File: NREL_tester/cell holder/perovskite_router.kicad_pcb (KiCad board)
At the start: 2 copper layers, 38.4 x 45.1 mm, 9 parts, among them J1 Conn_01x10_Male, J2 Conn_01x10_Male, U1 Perovskite_CP_6_Cell, U2 MCP9808_MSOP

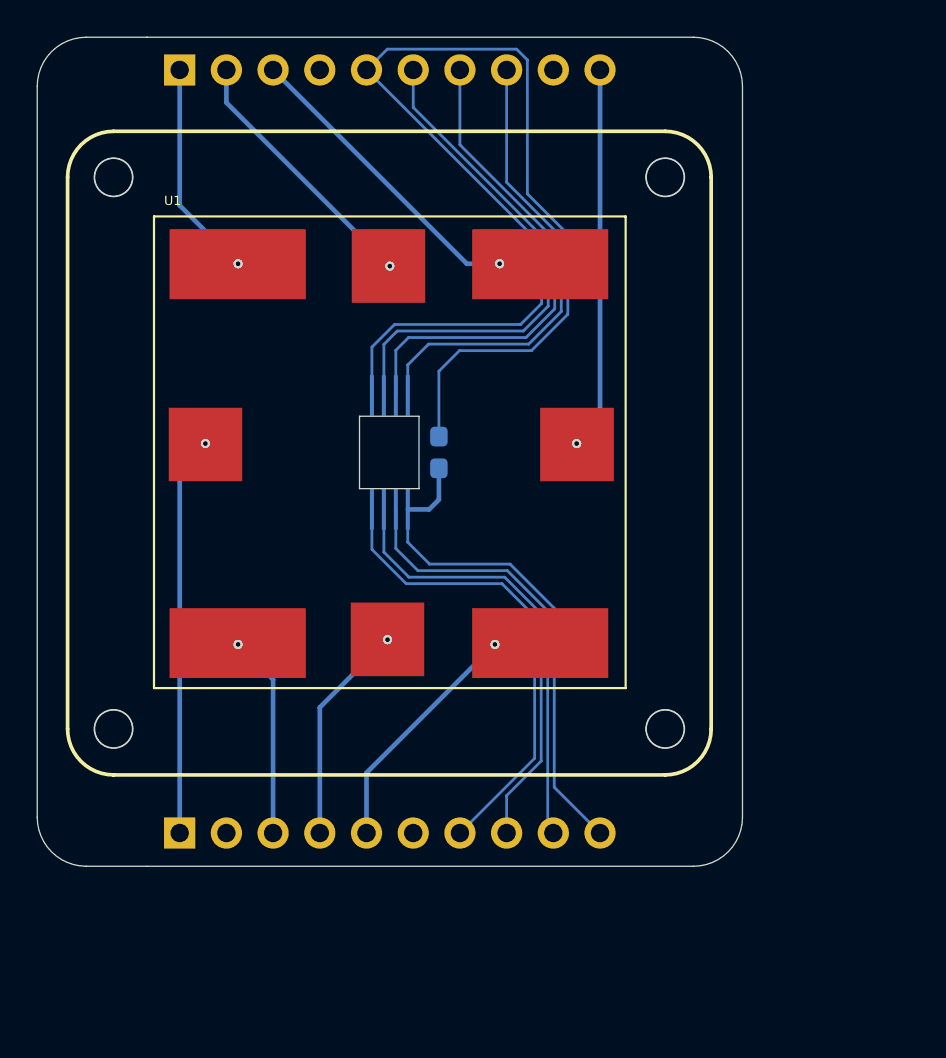
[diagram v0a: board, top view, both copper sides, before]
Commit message: Review contact board
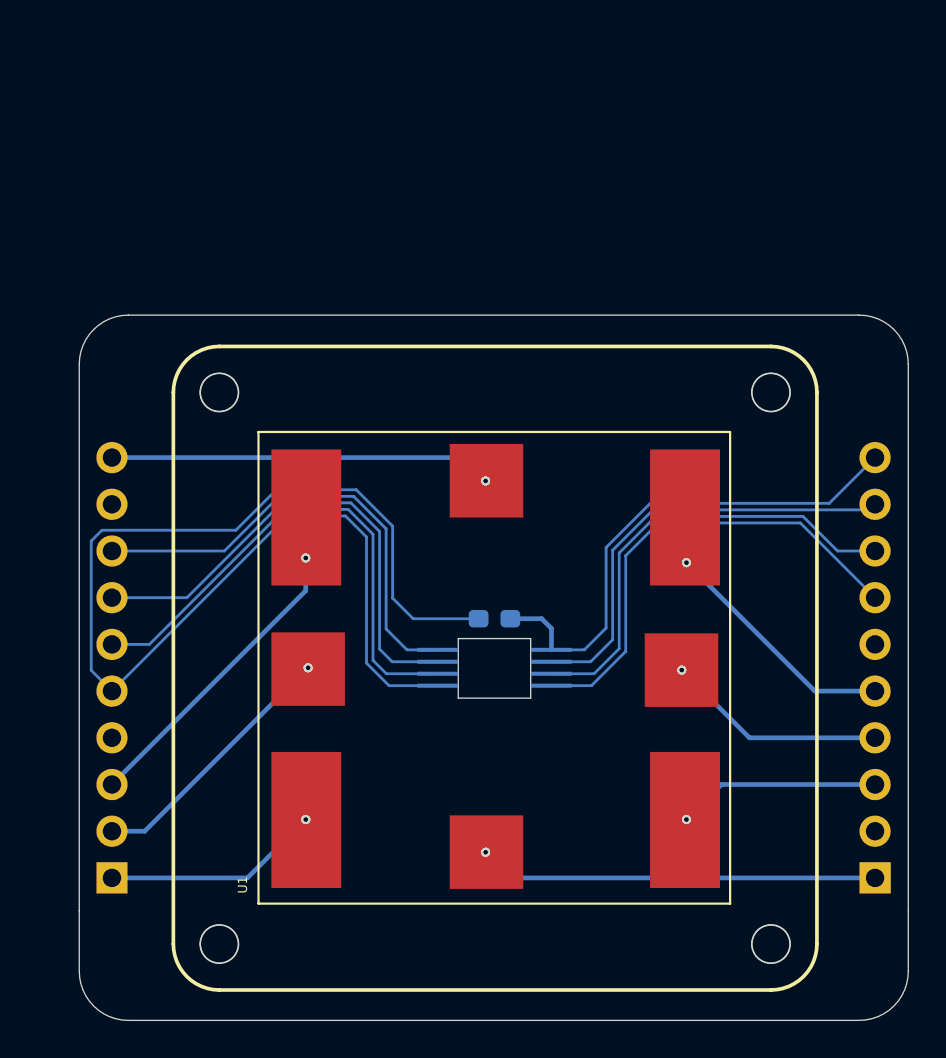
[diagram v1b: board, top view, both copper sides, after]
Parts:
- moved J1 44.1 mm to (134.4, 109.2), turned to 0 degrees
- moved REF** 42.1 mm to (140.2, 112.8), turned to 90 degrees
- moved J2 37.9 mm to (175.9, 109.2), turned to 0 degrees
- moved U1 37.8 mm to (142.3, 110.6), turned to 90 degrees
- moved REF** 37.6 mm to (170.2, 112.8), turned to 90 degrees
- moved REF** 26.9 mm to (140.2, 82.8), turned to 90 degrees
- moved REF** 19.2 mm to (170.2, 82.8), turned to 90 degrees
- moved U2 13.0 mm to (155.2, 97.8), turned to 180 degrees
- moved C1 9.53 mm to (155.2, 95.1), turned to 180 degrees
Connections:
- net Net-(C1-Pad1) renamed +3V3
- net Net-(C1-Pad2) renamed GND
- net Net-(J1-Pad1) renamed CELL_1
- net Net-(J1-Pad10) renamed COMMON_2
- net Net-(J1-Pad2) renamed CELL_2
- net Net-(J1-Pad3) renamed CELL_3
- net Net-(J1-Pad6) renamed ALERT
- net Net-(J1-Pad7) renamed SCL
- net Net-(J1-Pad8) renamed SDA
- net Net-(J2-Pad1) renamed COMMON_1
- net Net-(J2-Pad3) renamed CELL_6
- net Net-(J2-Pad4) renamed CELL_5
- net Net-(J2-Pad5) renamed CELL_4
- net Net-(J2-Pad7) renamed A2
- net Net-(J2-Pad8) renamed A1
- net Net-(J2-Pad9) renamed A0
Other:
- board size 38.4 x 45.1 mm -> 45.1 x 38.4 mm
